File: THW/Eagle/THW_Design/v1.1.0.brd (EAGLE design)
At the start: 50.6 x 182.7 mm, 34 parts, among them U1 ADA4091-2ARZ-RL

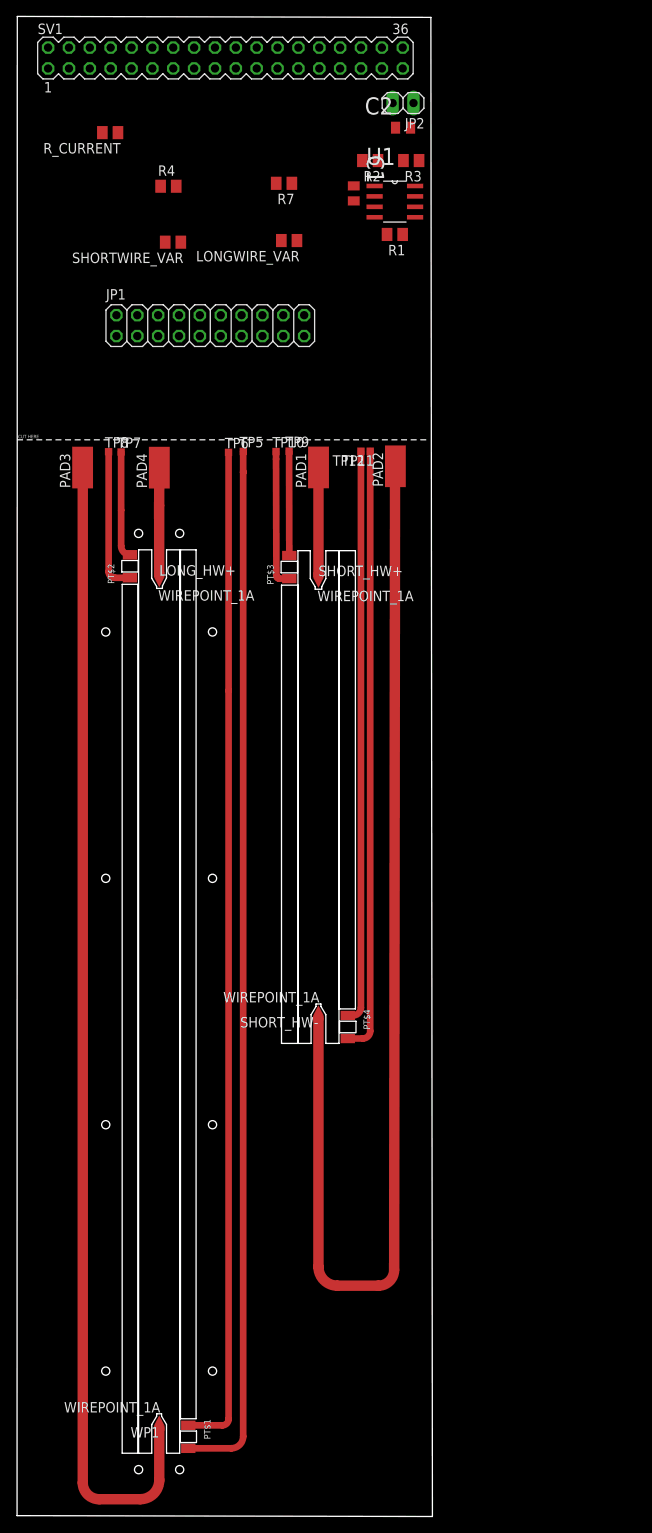
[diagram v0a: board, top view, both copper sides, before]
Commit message: new version
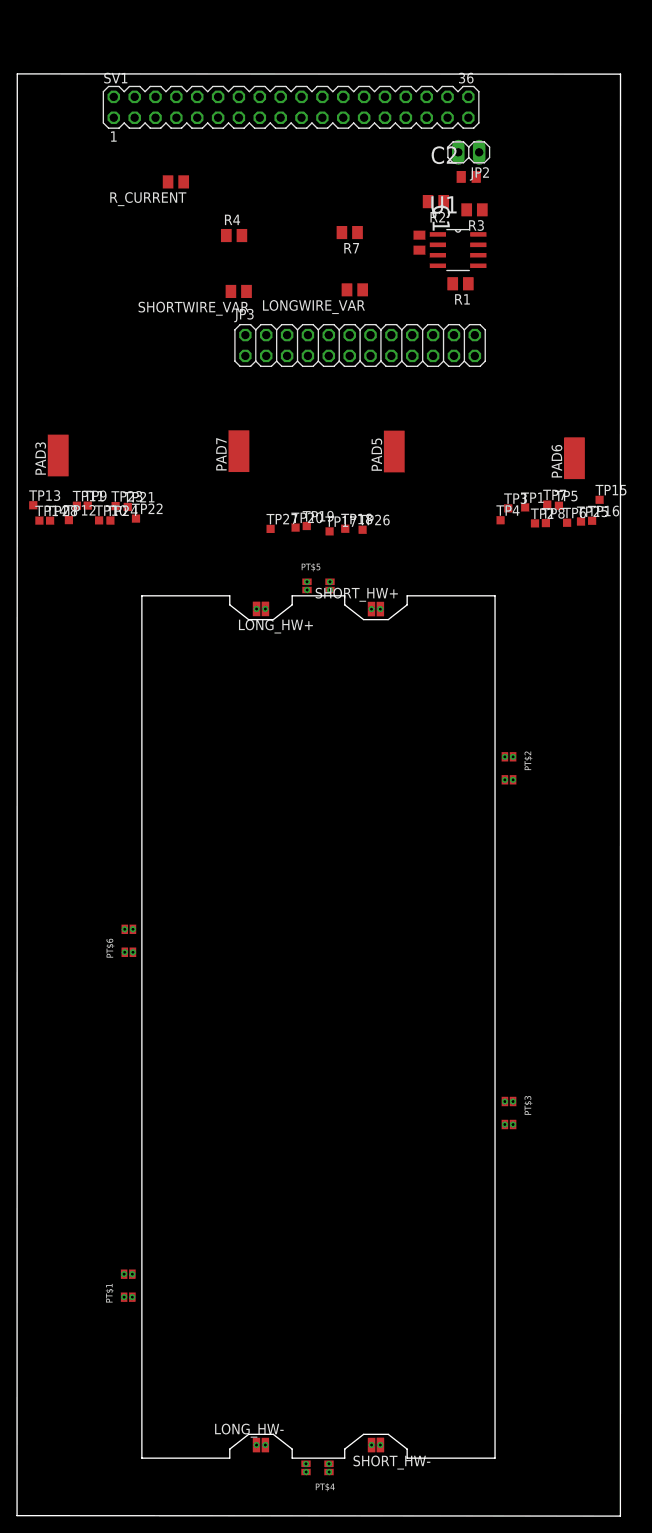
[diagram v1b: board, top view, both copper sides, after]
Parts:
- removed JP1: (no value), pinhead:2X10
- removed PAD1, PAD2, PAD4: (no value), wirepad:SMD2,54-5,08
- removed WP1: WIREPOINT_1A, WIREPOINT:WIREPOINT
- added JP3: (no value), pinhead:2X12
- added LONG_HW-: WIREPOINT_1A, WIREPOINT:WIREPOINT
- added PAD5, PAD6, PAD7: (no value), wirepad:SMD2,54-5,08
- added PT$5, PT$6: PTS1206A, PTS1206:CAPMP3216X166
- added TP1, TP13, TP14, TP15, TP16, TP17, TP18, TP19, TP2, TP20, TP21, TP22, TP23, TP24, TP25, TP26, TP27, TP28, TP3, TP4: TPTP10SQ, testpad:TP10SQ
- TP10, TP11, TP12, TP5, TP6, TP7, TP8, TP9: value TPSQTP09SQ -> TPTP10SQ; device testpad:TP09SQ -> testpad:TP10SQ
- moved PT$3 71.7 mm to (59.9, 49.0), turned to 270 degrees
- moved SHORT_HW- 54.7 mm to (43.7, 8.60), turned to 0 degrees
- moved TP8 53.9 mm to (64.4, 120.9)
- moved PT$4 53.8 mm to (36.6, 5.81), turned to 180 degrees
- moved PT$2 52.3 mm to (59.9, 91.0), turned to 270 degrees
- moved TP7 52.3 mm to (64.6, 123.1)
- moved TP6 42.1 mm to (67.0, 120.9)
- moved TP5 39.0 mm to (66.0, 123.0)
- moved TP12 36.5 mm to (6.31, 121.2), turned to 0 degrees
- moved TP11 36.3 mm to (7.29, 123.0), turned to 0 degrees
- moved TP9 25.4 mm to (8.61, 123.0)
- moved TP10 23.1 mm to (9.99, 121.2)
- moved PT$1 19.8 mm to (13.5, 28.0), turned to 90 degrees
- moved C1 10.0 mm to (49.0, 155.0)
- moved C2 10.0 mm to (55.0, 163.0)
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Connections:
- removed net T_S1+: JP1.1, PT$1.+, TP5.TP
- removed net T_S1-: JP1.2, PT$1.-, TP6.TP
- removed net T_S2+: JP1.3, PT$2.+, TP7.TP
- removed net T_S2-: JP1.4, PT$2.-, TP8.TP
- removed net T_S3+: JP1.5, PT$3.+, TP9.TP
- removed net T_S3-: JP1.6, PT$3.-, TP10.TP
- removed net T_S4+: JP1.7, PT$4.+, TP11.TP
- removed net T_S4-: JP1.8, PT$4.-, TP12.TP
- new net LONG_HW_SENS+: LONG_HW+.P$2, TP27.TP
- new net LONG_HW_SENS-: LONG_HW-.P$1, TP28.TP
- new net PT1_+: JP3.1, PT$2.+, TP1.TP
- new net PT1_-: JP3.2, PT$2.-, TP3.TP
- new net PT1_S+: JP3.3, PT$2.SENS+, TP2.TP
- new net PT1_S-: JP3.4, PT$2.SENS-, TP4.TP
- new net PT2_+: JP3.5, PT$3.+, TP5.TP
- new net PT2_-: JP3.6, PT$3.-, TP7.TP
- new net PT2_S+: JP3.7, PT$3.SENS+, TP6.TP
- new net PT2_S-: JP3.8, PT$3.SENS-, TP8.TP
- new net PT3_+: JP3.9, PT$1.+, TP9.TP
- new net PT3_-: JP3.10, PT$1.-, TP11.TP
- new net PT3_S+: JP3.11, PT$1.SENS+, TP10.TP
- new net PT3_S-: JP3.12, PT$1.SENS-, TP12.TP
- new net PT4_+: JP3.13, PT$4.+, TP13.TP
- new net PT4_-: JP3.14, PT$4.-, TP15.TP
- new net PT4_S+: JP3.15, PT$4.SENS+, TP14.TP
- new net PT4_S-: JP3.16, PT$4.SENS-, TP16.TP
- new net PT5_+: JP3.17, PT$5.+, TP17.TP
- new net PT5_-: JP3.18, PT$5.-, TP19.TP
- new net PT5_S+: JP3.19, PT$5.SENS+, TP18.TP
- new net PT5_S-: JP3.20, PT$5.SENS-, TP20.TP
- new net PT6_+: JP3.21, PT$6.+, TP21.TP
- new net PT6_-: JP3.22, PT$6.-, TP23.TP
- new net PT6_S+: JP3.23, PT$6.SENS+, TP22.TP
- new net PT6_S-: JP3.24, PT$6.SENS-, TP24.TP
- new net SHORT_HW_SENS+: SHORT_HW+.P$2, TP26.TP
- new net SHORT_HW_SENS-: SHORT_HW-.P$1, TP25.TP
- net LONG_HW+: now also PAD7.1; no longer PAD4.1, SV1.1
- net LONG_HW-: now also LONG_HW-.P$2; no longer SV1.2, WP1.P$1
- net SHORT_HW+: now also PAD5.1; no longer PAD1.1, SV1.35
- net SHORT_HW-: now also PAD6.1, SHORT_HW-.P$2; no longer PAD2.1, SHORT_HW-.P$1, SV1.36
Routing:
- net PT4_+: track 0.00 -> 151.2 mm, vias 0 -> 1
- net PT4_-: track 0.00 -> 151.1 mm, vias 0 -> 1
- net PT4_S+: track 0.00 -> 149.6 mm, vias 0 -> 1
- net PT4_S-: track 0.00 -> 148.4 mm, vias 0 -> 1
- net LONG_HW_SENS-: track 0.00 -> 142.5 mm, vias 0 -> 1
- net SHORT_HW_SENS-: track 0.00 -> 141.4 mm, vias 0 -> 1
- net T_S1+: track 127.4 -> 0.00 mm
- net T_S1-: track 122.9 -> 0.00 mm
- net PT3_S-: track 0.00 -> 100.8 mm, vias 0 -> 1
- net PT3_-: track 0.00 -> 97.6 mm, vias 0 -> 1
- net PT3_+: track 0.00 -> 93.8 mm, vias 0 -> 1
- net PT3_S+: track 0.00 -> 92.7 mm, vias 0 -> 1
- net PT2_S+: track 0.00 -> 81.0 mm, vias 0 -> 1
- net PT2_+: track 0.00 -> 76.2 mm, vias 0 -> 1
- net T_S4+: track 73.7 -> 0.00 mm
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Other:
- board size 50.6 x 182.7 mm -> 73.5 x 175.6 mm
- board text removed: "CUT HERE"
- board text removed: "R = 0.00498"
- board text removed: "R = 0.00502"
- board text removed: "R = 0.00760"
- board text removed: "R = 0.00784"
- board text removed: "R = 0.0101"
- board text removed: "R = 0.0103"
- board text removed: "R = 0.0418"
- board text removed: "R = 0.0441"
- board text removed: "R = 0.0535"
- board text removed: "R = 0.0542"
- board text removed: "R = 0.0735"
- board text removed: "R = 0.0763"
